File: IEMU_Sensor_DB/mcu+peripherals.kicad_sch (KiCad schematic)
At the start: 34 parts, among them J201 Conn_ARM_SWD_TagConnect_TC203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, U201 Ezurio BL54L15, U202 W25N02JWZEIF, U203 LSM6DSV320XTR, U204 MMC5603NJ, Y201 32.768kHz

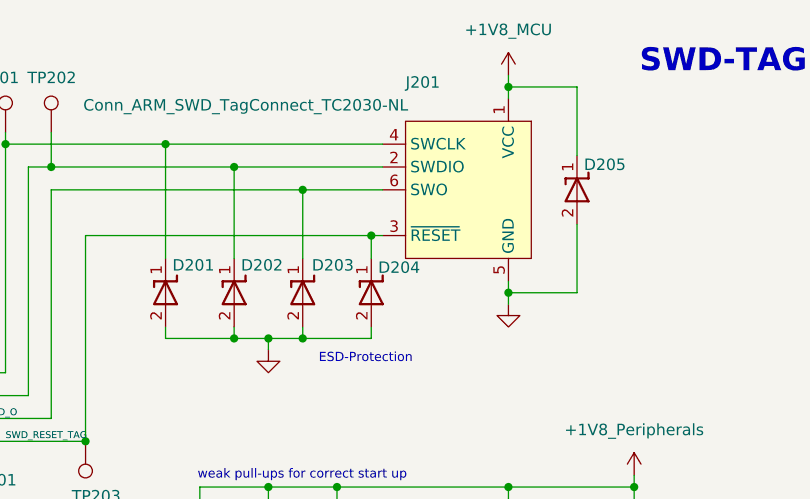
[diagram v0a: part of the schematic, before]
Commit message: commit after component purchase
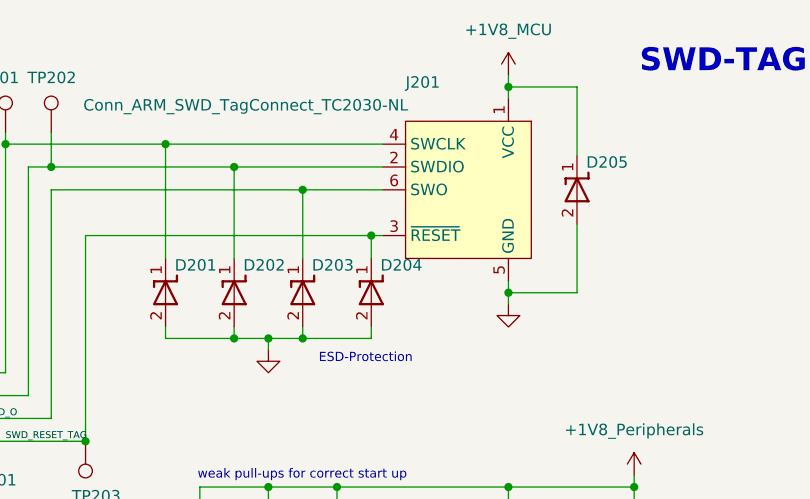
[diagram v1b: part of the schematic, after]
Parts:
- removed D201, D202, D203, D204, D205: ESD9L1P8, Diode_SMD:D_SOD-882, symbol 0_Power:ESD9L1P8
- added D201, D202, D203, D204, D205: RCLAMP01811PW.C, 0_Power:DIODFN100X60X55-2N, symbol 0_Power:RCLAMP01811PW.C
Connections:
- net +1V8_MCU: now also D205.1 (I/O)
- net GND: now also D201.2 (GND), D202.2 (GND), D203.2 (GND), D204.2 (GND), D205.2 (GND)
- net SWD_CLK: now also D201.1 (I/O)
- net SWD_IO: now also D202.1 (I/O)
- net SWD_O: now also D203.1 (I/O)
- net SWD_RESET_TAG: now also D204.1 (I/O)
